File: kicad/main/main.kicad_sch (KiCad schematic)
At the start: 15 parts, among them J1 XT60F, J2 XT60M, M1 NEMA 8 Bipolar Stepper, M2 HSR-2648CR, SW1 L101011_SPST, U1 A4988, U2 S13V10F5, U3 BeagleBone Black Wireless, U4 BNO055

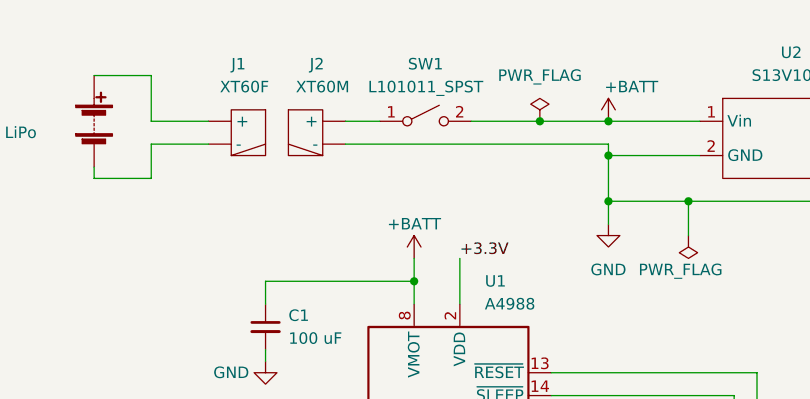
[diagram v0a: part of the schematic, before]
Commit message: Updated all schematics
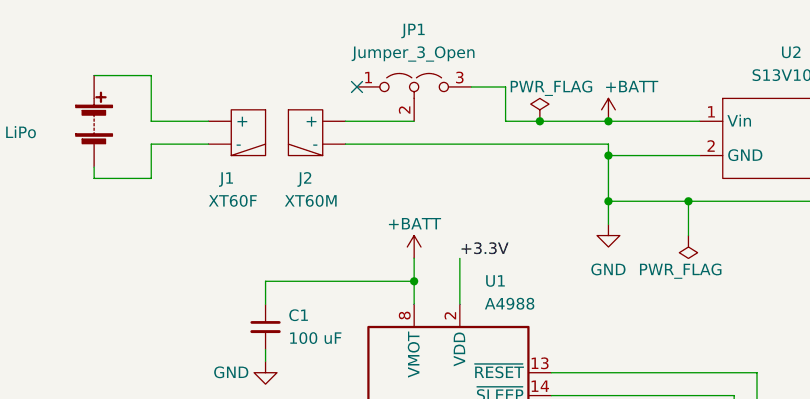
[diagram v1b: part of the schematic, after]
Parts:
- removed SW1: L101011_SPST, symbol Switch:SW_SPST
- added JP1: Jumper_3_Open, symbol Jumper:Jumper_3_Open
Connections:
- net +BATT: now also JP1.3 (B)
- new net: J2. (-), JP1.2 (C)
- no-connect marks 8 -> 9
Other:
- company: (none) -> Peter Costescu
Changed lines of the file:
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@@
     (title "Payload Main Subsystem")
     (date "2022-12-30")
-    (rev "1.7")
+    (rev "1.8")
+    (company "Peter Costescu")
   )
   (junction (at 95.25 27.94) (diameter 0) (color 0 0 0 0)
@@
   (junction (at 162.56 52.07) (diameter 0) (color 0 0 0 0)
   )
+  (junction (at 87.63 24.13) (diameter 0) (color 0 0 0 0)
+  )
   (junction (at 73.66 83.82) (diameter 0) (color 0 0 0 0)
   )
@@
   )
   (junction (at 167.64 67.31) (diameter 0) (color 0 0 0 0)
-  )
-  (junction (at 87.63 24.13) (diameter 0) (color 0 0 0 0)
   )
   (junction (at 137.16 24.13) (diameter 0) (color 0 0 0 0)
@@
   (no_connect (at 88.9 69.85))
   (no_connect (at 88.9 74.93))
+  (no_connect (at 67.31 20.32))
   (no_connect (at 191.77 69.85))
   (no_connect (at 88.9 59.69))
@@
     (stroke (width 0) (type default) (color 0 0 0 0))
   )
+  (wire (pts (xy 83.82 24.13) (xy 87.63 24.13))
+    (stroke (width 0) (type default) (color 0 0 0 0))
+  )
   (wire (pts (xy 114.3 73.66) (xy 114.3 88.9))
     (stroke (width 0) (type default) (color 0 0 0 0))
@@
     (stroke (width 0) (type default) (color 0 0 0 0))
   )
+  (wire (pts (xy 83.82 20.32) (xy 83.82 24.13))
+    (stroke (width 0) (type default) (color 0 0 0 0))
+  )
   (wire (pts (xy 109.22 64.77) (xy 116.84 64.77))
     (stroke (width 0) (type default) (color 0 0 0 0))
@@
     (stroke (width 0) (type default) (color 0 0 0 0))
   )
-  (wire (pts (xy 80.01 24.13) (xy 87.63 24.13))
-    (stroke (width 0) (type default) (color 0 0 0 0))
-  )
   (wire (pts (xy 88.9 64.77) (xy 104.14 64.77))
     (stroke (width 0) (type default) (color 0 0 0 0))
@@
     (stroke (width 0) (type default) (color 0 0 0 0))
   )
-  (wire (pts (xy 66.04 24.13) (xy 69.85 24.13))
-    (stroke (width 0) (type default) (color 0 0 0 0))
-  )
   (wire (pts (xy 160.02 52.07) (xy 162.56 52.07))
     (stroke (width 0) (type default) (color 0 0 0 0))
@@
     (stroke (width 0) (type default) (color 0 0 0 0))
   )
+  (wire (pts (xy 66.04 24.13) (xy 73.66 24.13))
+    (stroke (width 0) (type default) (color 0 0 0 0))
+  )
   (wire (pts (xy 66.04 59.69) (xy 44.45 59.69))
     (stroke (width 0) (type default) (color 0 0 0 0))
   )
+  (wire (pts (xy 80.01 20.32) (xy 83.82 20.32))
+    (stroke (width 0) (type default) (color 0 0 0 0))
+  )
   (wire (pts (xy 49.53 74.93) (xy 55.88 74.93))
     (stroke (width 0) (type default) (color 0 0 0 0))
@@
     (stroke (width 0) (type default) (color 0 0 0 0))
   )
-  (image (at 133.35 111.76)
+  (image (at 143.51 111.76)
     (data
       iVBORw0KGgoAAAANSUhEUgAAAbIAAACKCAYAAADPLc9oAAAABHNCSVQICAgIfAhkiAAAAAlwSFlz
@@
   (symbol (lib_id "power:GND") (at 170.18 76.2 0) (unit 1)
     (in_bom yes) (on_board yes) (fields_autoplaced)
-    (property "Reference" "#PWR08" (id 0) (at 170.18 82.55 0)
+    (property "Reference" "#PWR09" (id 0) (at 170.18 82.55 0)
       (effects (font (size 1.27 1.27)) hide)
     )
@@
   (symbol (lib_id "payload_symbol_library:XT60M") (at 59.69 22.86 0) (unit 1)
     (in_bom yes) (on_board yes)
-    (property "Reference" "J2" (id 0) (at 62.865 17.78 0))
-    (property "Value" "XT60M" (id 1) (at 63.5 20.32 0))
+    (property "Reference" "J2" (id 0) (at 61.595 30.48 0))
+    (property "Value" "XT60M" (id 1) (at 62.23 33.02 0))
     (property "Footprint" "" (id 2) (at 59.69 22.86 0)
       (effects (font (size 1.27 1.27)) hide)
@@
   (symbol (lib_id "payload_symbol_library:XT60F") (at 57.15 24.13 0) (mirror y) (unit 1)
     (in_bom yes) (on_board yes)
-    (property "Reference" "J1" (id 0) (at 53.34 17.78 0)
+    (property "Reference" "J1" (id 0) (at 52.07 30.48 0)
       (effects (font (size 1.27 1.27)) (justify right))
     )
-    (property "Value" "XT60F" (id 1) (at 52.07 20.32 0)
+    (property "Value" "XT60F" (id 1) (at 50.8 33.02 0)
       (effects (font (size 1.27 1.27)) (justify right))
     )
@@
   )
   (symbol (lib_id "power:PWR_FLAG") (at 87.63 24.13 0) (unit 1)
-    (in_bom yes) (on_board yes) (fields_autoplaced)
+    (in_bom yes) (on_board yes)
     (property "Reference" "#FLG01" (id 0) (at 87.63 22.225 0)
       (effects (font (size 1.27 1.27)) hide)
     )
-    (property "Value" "PWR_FLAG" (id 1) (at 87.63 19.05 0))
+    (property "Value" "PWR_FLAG" (id 1) (at 88.9 20.32 0))
     (property "Footprint" "" (id 2) (at 87.63 24.13 0)
       (effects (font (size 1.27 1.27)) hide)
@@
     (pin "1")
   )
+  (symbol (lib_id "Jumper:Jumper_3_Open") (at 73.66 20.32 0) (unit 1)
+    (in_bom yes) (on_board yes) (fields_autoplaced)
+    (property "Reference" "JP1" (id 0) (at 73.66 13.97 0))
+    (property "Value" "Jumper_3_Open" (id 1) (at 73.66 16.51 0))
+    (property "Footprint" "" (id 2) (at 73.66 20.32 0)
+      (effects (font (size 1.27 1.27)) hide)
+    )
+    (property "Datasheet" "~" (id 3) (at 73.66 20.32 0)
+      (effects (font (size 1.27 1.27)) hide)
+    )
+    (pin "1")
+    (pin "2")
+    (pin "3")
+  )
   (symbol (lib_id "power:GND") (at 144.78 31.75 0) (unit 1)
     (in_bom yes) (on_board yes) (fields_autoplaced)
-    (property "Reference" "#PWR09" (id 0) (at 144.78 38.1 0)
+    (property "Reference" "#PWR08" (id 0) (at 144.78 38.1 0)
       (effects (font (size 1.27 1.27)) hide)
     )
@@
     (pin "2")
   )
-  (symbol (lib_id "Switch:SW_SPST") (at 74.93 24.13 0) (unit 1)
-    (in_bom yes) (on_board yes) (fields_autoplaced)
-    (property "Reference" "SW1" (id 0) (at 74.93 17.78 0))
-    (property "Value" "L101011_SPST" (id 1) (at 74.93 20.32 0))
-    (property "Footprint" "" (id 2) (at 74.93 24.13 0)
-      (effects (font (size 1.27 1.27)) hide)
-    )
-    (property "Datasheet" "~" (id 3) (at 74.93 24.13 0)
-      (effects (font (size 1.27 1.27)) hide)
-    )
-    (pin "1")
-    (pin "2")
-  )
   (symbol (lib_id "power:+BATT") (at 128.27 90.17 0) (unit 1)
     (in_bom yes) (on_board yes)
@@
       (reference "#PWR07") (unit 1) (value "+BATT") (footprint "")
     )
+    (path "/9d1c4416-be2b-4534-959b-8aaef2b0de36"
+      (reference "#PWR08") (unit 1) (value "GND") (footprint "")
+    )
     (path "/37de6bbb-6273-4906-807b-25c12386cb60"
-      (reference "#PWR08") (unit 1) (value "GND") (footprint "")
-    )
-    (path "/9d1c4416-be2b-4534-959b-8aaef2b0de36"
       (reference "#PWR09") (unit 1) (value "GND") (footprint "")
     )
@@
       (reference "J2") (unit 1) (value "XT60M") (footprint "")
     )
+    (path "/9c0488df-4fbe-4ed4-a042-48cd58c8b662"
+      (reference "JP1") (unit 1) (value "Jumper_3_Open") (footprint "")
+    )
     (path "/c539e74f-c9b8-43cc-9641-ae0b6f11b03b"
       (reference "M1") (unit 1) (value "NEMA 8 Bipolar Stepper") (footprint "")
@@
       (reference "R2") (unit 1) (value "5.6K") (footprint "")
     )
-    (path "/e73ec205-4335-431a-bc86-dab5f72536c8"
-      (reference "SW1") (unit 1) (value "L101011_SPST") (footprint "")
-    )
     (path "/b49d0fa0-778f-4fbe-8301-0095ef3304a9"
